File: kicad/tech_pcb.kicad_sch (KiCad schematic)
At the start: 24 parts, among them J1 Conn_01x11, J2 Conn_01x11, J3 USB_C_Receptacle_USB2.0_16P, J4 Conn_01x03_MountingPin, SW1 RST, SW2 BOOT, U1 STM32C071GBUxN, U2 XC6206PxxxMR

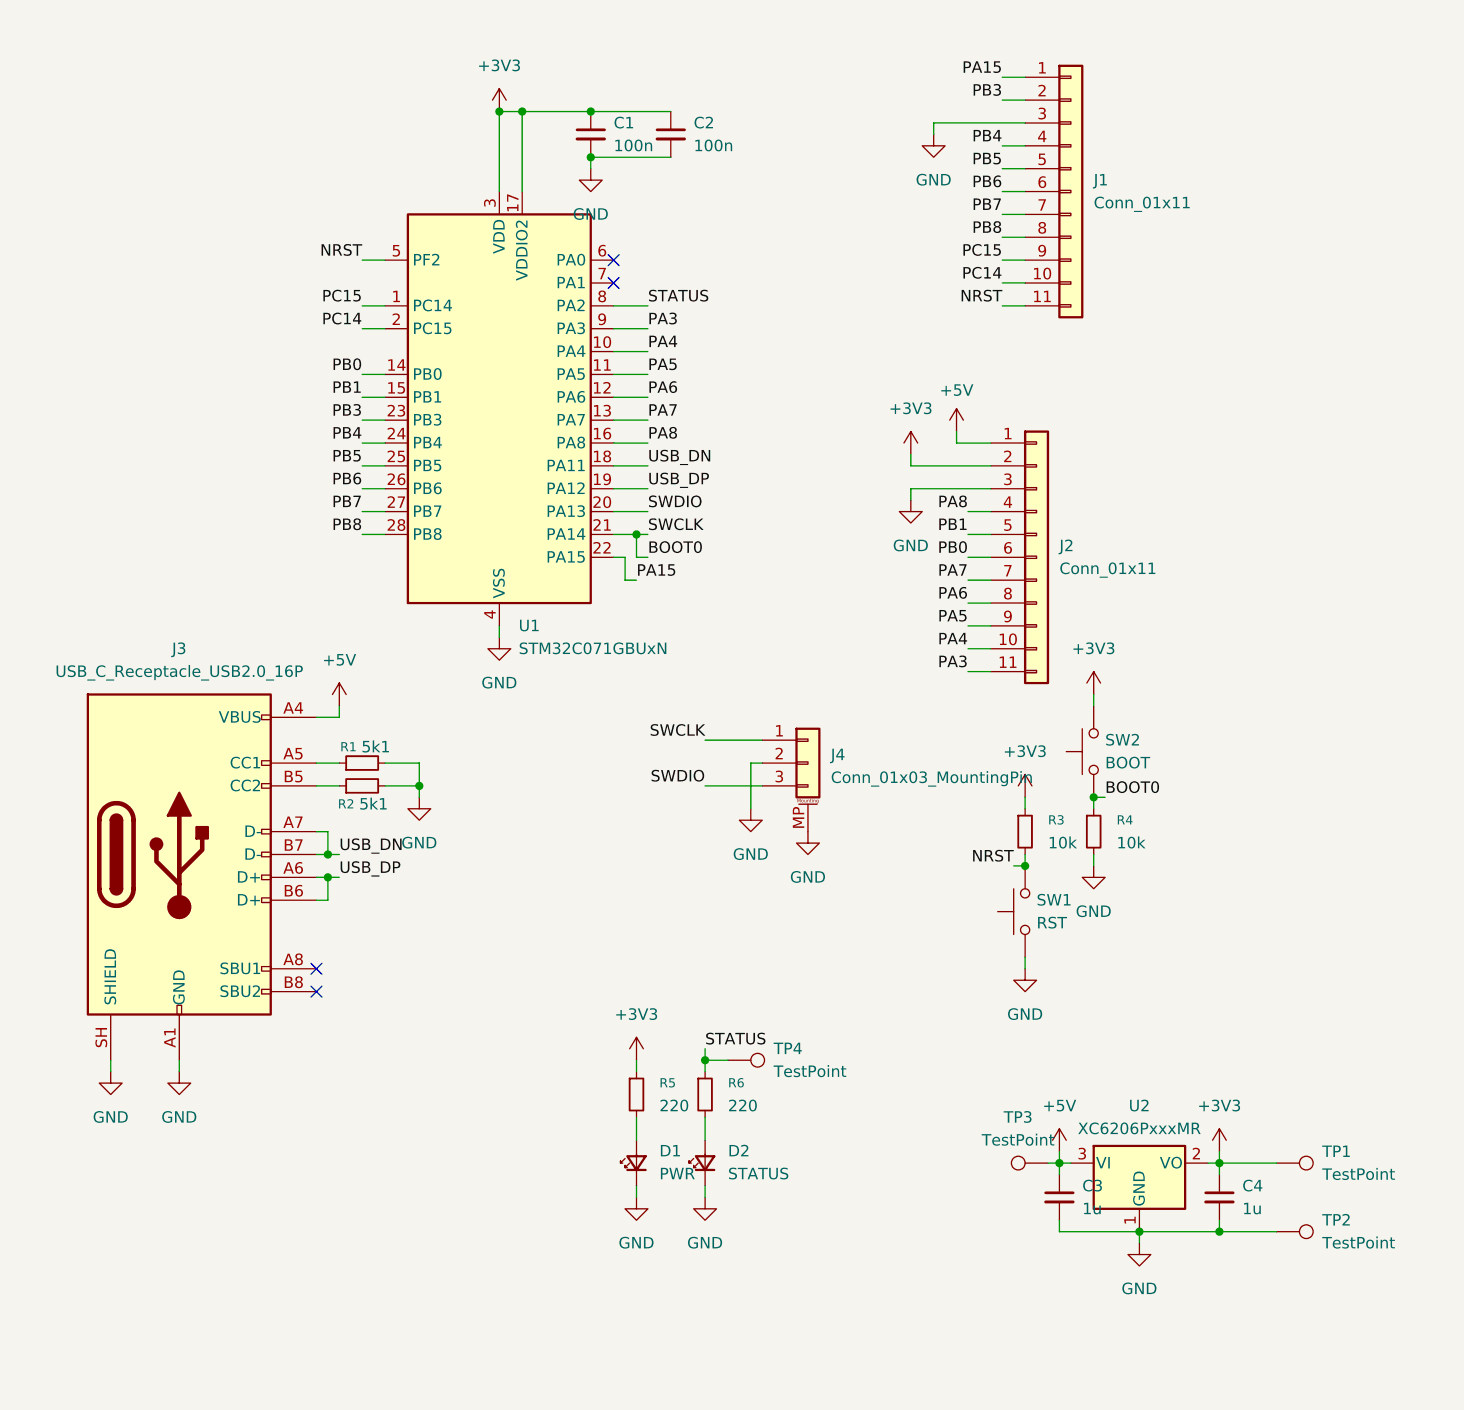
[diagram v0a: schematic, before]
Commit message: Tidy up the schematic
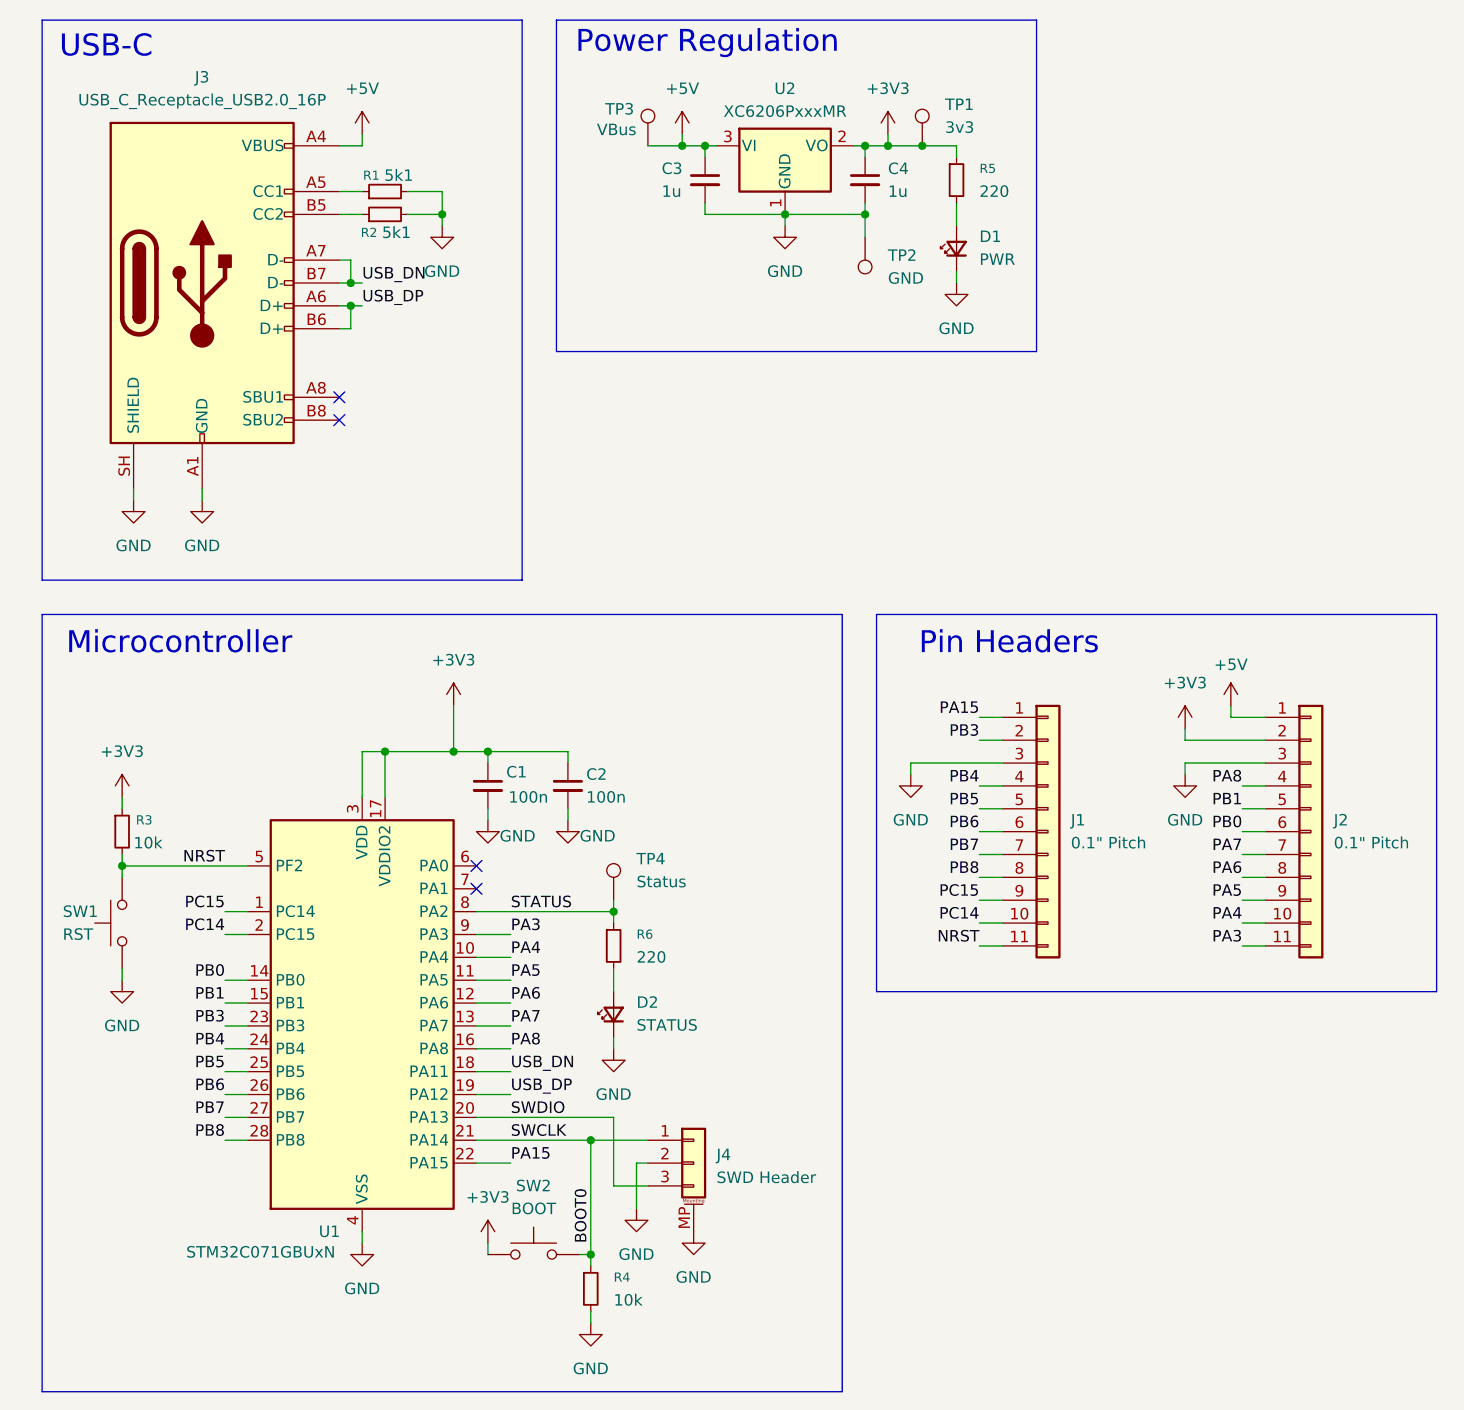
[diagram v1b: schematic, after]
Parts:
- J1, J2: value Conn_01x11 -> 0.1" Pitch
- J4: value Conn_01x03_MountingPin -> SWD Header
- TP1: value TestPoint -> 3v3
- TP2: value TestPoint -> GND
- TP3: value TestPoint -> VBus
- TP4: value TestPoint -> Status
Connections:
- net +3V3: now also SW2.1; no longer SW2.2
- net BOOT0: now also SW2.2; no longer SW2.1
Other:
- note added: "Microcontroller"
- note added: "Pin Headers"
- note added: "Power Regulation"
- note added: "USB-C"
- company: (none) -> Tennessee Technological University
- title: (none) -> TN Tech PCB Design Workshop
- moved on the sheet: C1, C2, C3, C4, D1, D2, J1, J2, J3, J4, R1, R2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
